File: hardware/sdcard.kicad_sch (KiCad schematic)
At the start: 18 parts

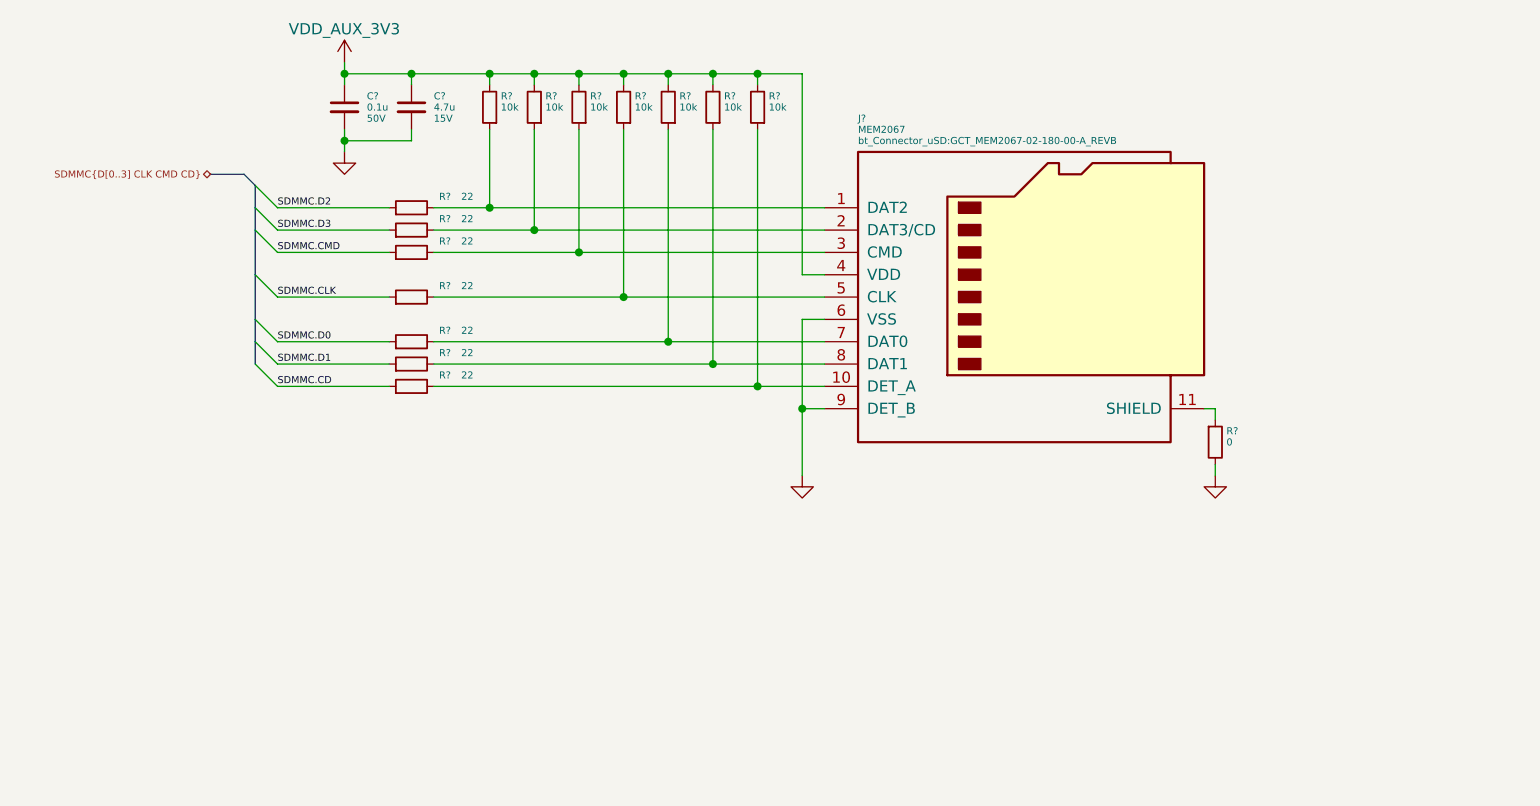
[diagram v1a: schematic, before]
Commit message: ready for first review
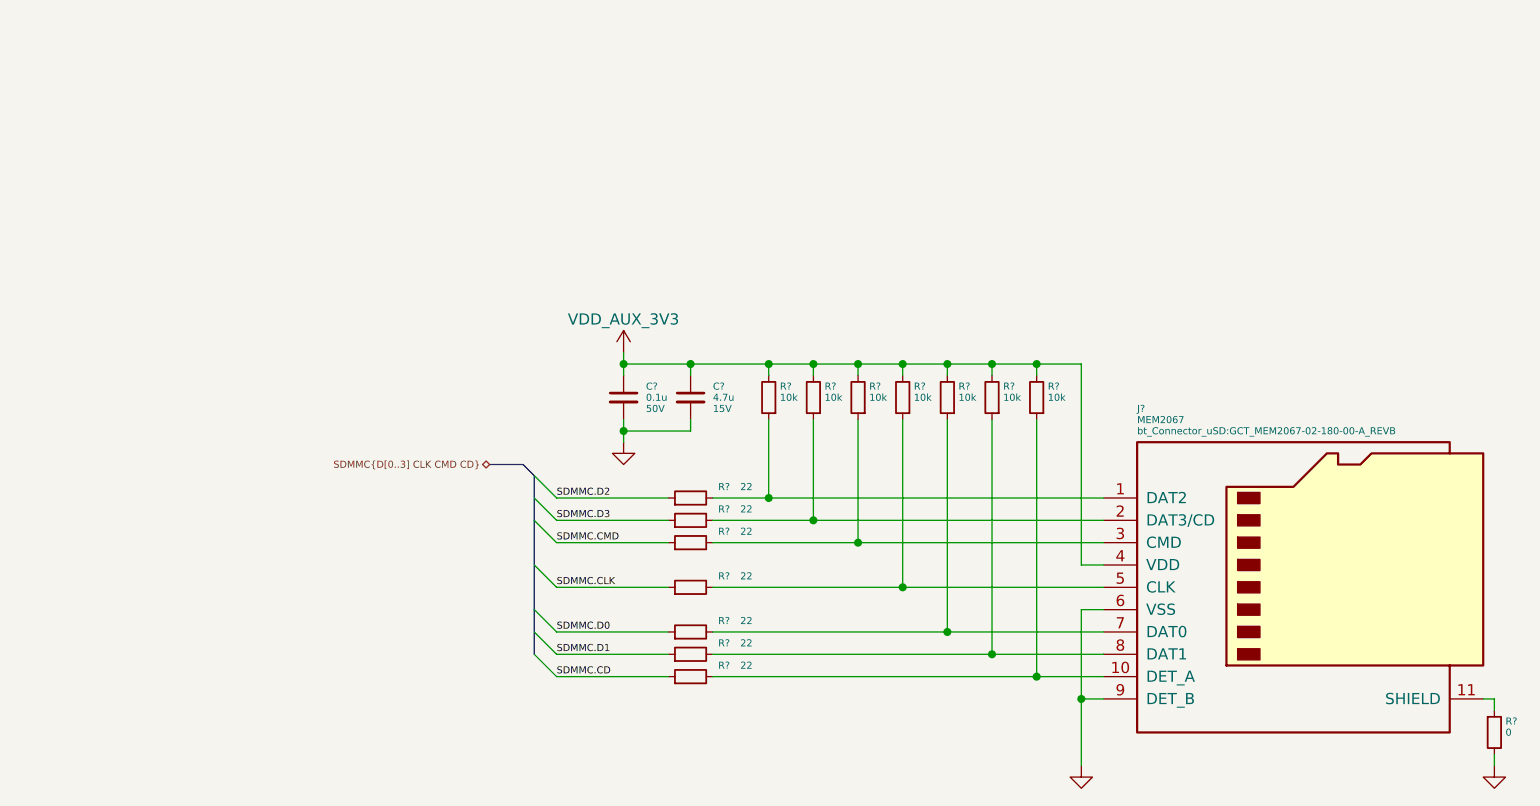
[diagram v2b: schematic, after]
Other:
- moved on the sheet: C?, J?, R?
